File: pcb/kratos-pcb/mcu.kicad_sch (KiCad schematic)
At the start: 1 part, among them U1 ESP32-DEVKIT-V1

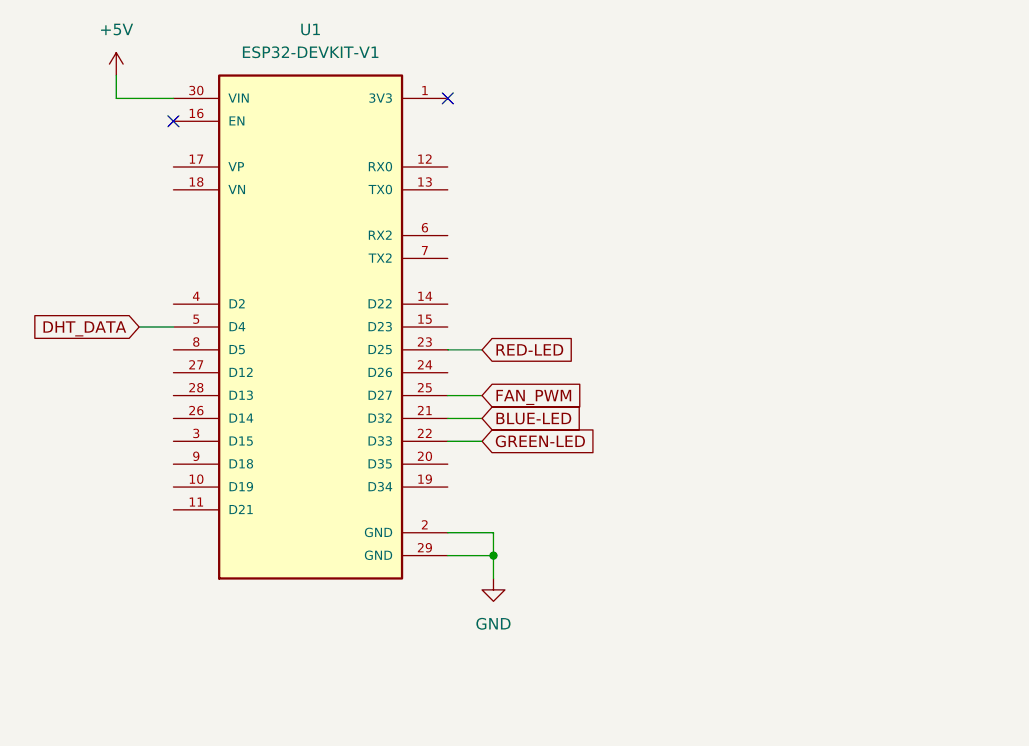
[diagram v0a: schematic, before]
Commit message: ### added
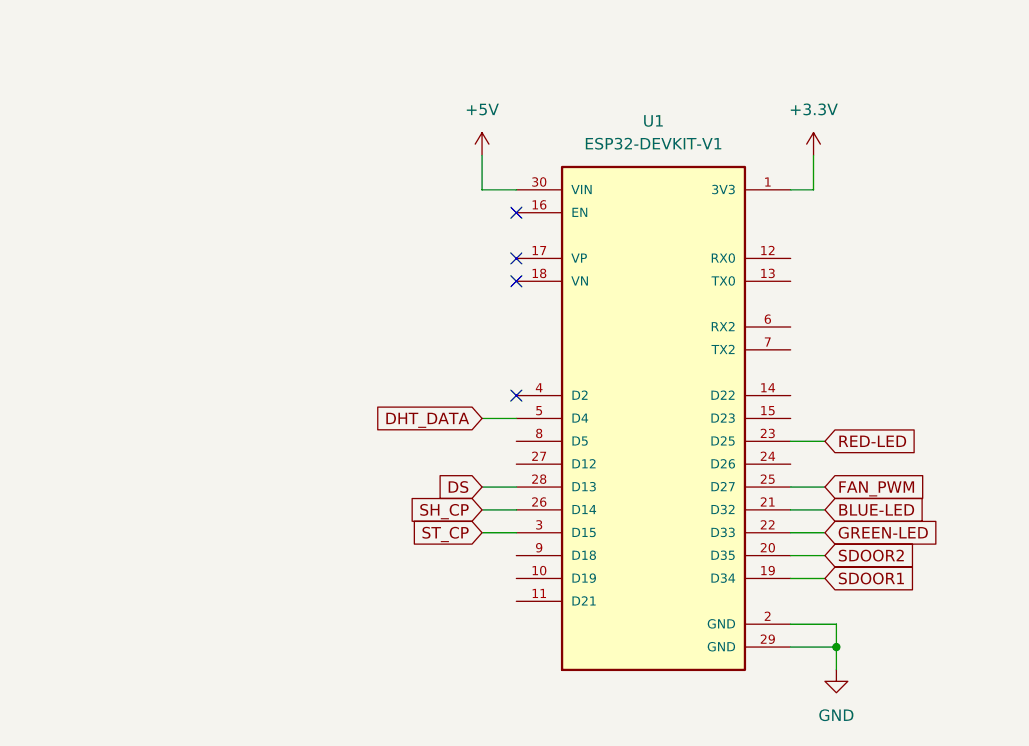
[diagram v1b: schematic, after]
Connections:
- net +3.3V: now reaches U1.1 (3V3)
- net SDOOR1: now reaches U1.19 (D34)
- net SDOOR2: now reaches U1.20 (D35)
- net SH_CP: now reaches U1.26 (D14)
- net DS: now reaches U1.28 (D13)
- net ST_CP: now reaches U1.3 (D15)
- no-connect marks 2 -> 4
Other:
- moved on the sheet: U1

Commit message: ### update     - kicad schematic
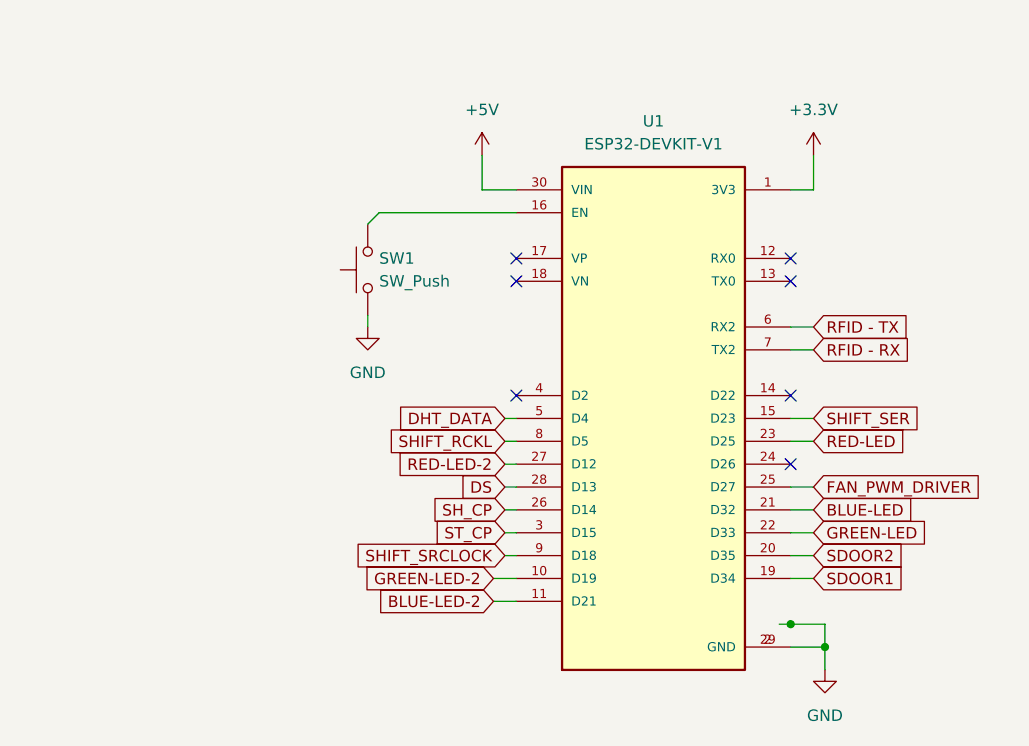
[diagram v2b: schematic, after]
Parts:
- added SW1: SW_Push, Button_Switch_THT:SW_PUSH_6mm_H4.3mm, symbol Switch:SW_Push
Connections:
- net GND: now also SW1.1
- net GREEN-LED-2: now reaches U1.10 (D19)
- net BLUE-LED-2: now reaches U1.11 (D21)
- net SHIFT_SER: now reaches U1.15 (D23)
- net at U1.16 (EN): now also SW1.2
- net RED-LED-2: now reaches U1.27 (D12)
- net RFID - TX: now reaches U1.6 (RX2)
- net RFID - RX: now reaches U1.7 (TX2)
- net SHIFT_RCKL: now reaches U1.8 (D5)
- net SHIFT_SRCLOCK: now reaches U1.9 (D18)
- net FAN_PWM renamed FAN_PWM_DRIVER
- no-connect marks 4 -> 7

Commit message: kicad
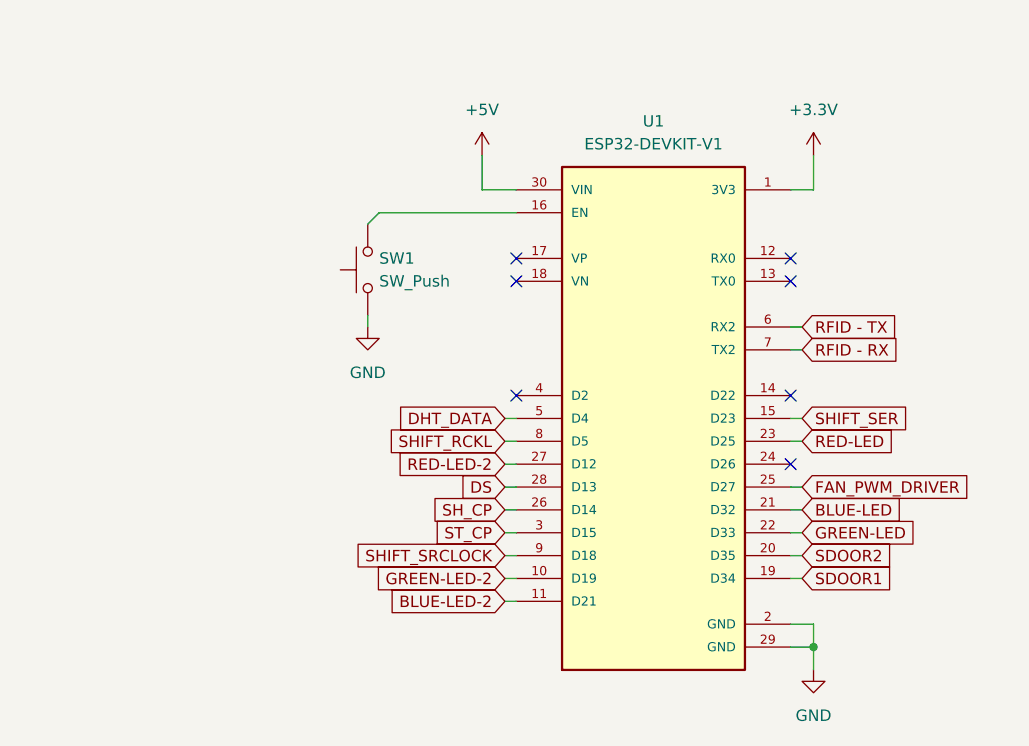
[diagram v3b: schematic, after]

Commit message: ### MODIFY
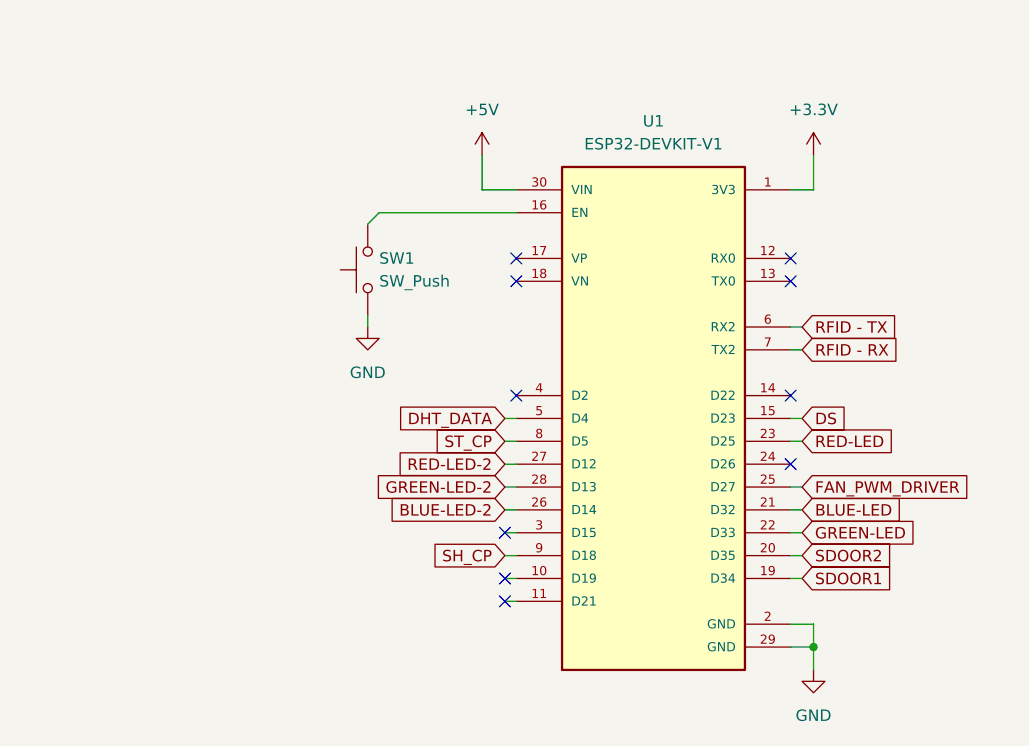
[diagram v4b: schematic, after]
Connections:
- net SHIFT_RCKL is gone; now on net ST_CP: U1.8 (D5)
- net SHIFT_SER is gone; now on net DS: U1.15 (D23)
- net SHIFT_SRCLOCK is gone; now on net SH_CP: U1.9 (D18)
- net BLUE-LED-2: now also U1.26 (D14); no longer U1.11 (D21)
- net DS: no longer U1.28 (D13)
- net GREEN-LED-2: now also U1.28 (D13); no longer U1.10 (D19)
- net SH_CP: no longer U1.26 (D14)
- net ST_CP: no longer U1.3 (D15)
- no-connect marks 7 -> 10
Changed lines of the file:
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@@
   (no_connect (at 158.75 101.6))
   (no_connect (at 128.27 78.74))
+  (no_connect (at 127 109.22))
+  (no_connect (at 127 114.3))
+  (no_connect (at 127 116.84))
   (no_connect (at 158.75 78.74))
   (no_connect (at 128.27 81.28))
@@
     (stroke (width 0) (type default))
   )
-  (global_label "SHIFT_SER" (shape input) (at 160.02 96.52 0) (fields_autoplaced)
-    (effects (font (size 1.27 1.27)) (justify left))
-    (property "Intersheetrefs" "${INTERSHEET_REFS}" (at 172.8023 96.52 0)
-      (effects (font (size 1.27 1.27)) (justify left) hide)
-    )
-  )
   (global_label "SDOOR2" (shape input) (at 160.02 111.76 0) (fields_autoplaced)
     (effects (font (size 1.27 1.27)) (justify left))
@@
     )
   )
-  (global_label "GREEN-LED-2" (shape input) (at 127 114.3 180) (fields_autoplaced)
+  (global_label "SH_CP" (shape input) (at 127 111.76 180) (fields_autoplaced)
     (effects (font (size 1.27 1.27)) (justify right))
-    (property "Intersheetrefs" "${INTERSHEET_REFS}" (at 110.0449 114.3 0)
+    (property "Intersheetrefs" "${INTERSHEET_REFS}" (at 117.9672 111.76 0)
       (effects (font (size 1.27 1.27)) (justify right) hide)
     )
   )
-  (global_label "SH_CP" (shape input) (at 127 106.68 180) (fields_autoplaced)
+  (global_label "BLUE-LED-2" (shape input) (at 127 106.68 180) (fields_autoplaced)
     (effects (font (size 1.27 1.27)) (justify right))
-    (property "Intersheetrefs" "${INTERSHEET_REFS}" (at 117.9672 106.68 0)
+    (property "Intersheetrefs" "${INTERSHEET_REFS}" (at 111.4358 106.68 0)
       (effects (font (size 1.27 1.27)) (justify right) hide)
     )
   )
-  (global_label "BLUE-LED-2" (shape input) (at 127 116.84 180) (fields_autoplaced)
+  (global_label "GREEN-LED-2" (shape input) (at 127 104.14 180) (fields_autoplaced)
     (effects (font (size 1.27 1.27)) (justify right))
-    (property "Intersheetrefs" "${INTERSHEET_REFS}" (at 111.4358 116.84 0)
+    (property "Intersheetrefs" "${INTERSHEET_REFS}" (at 110.0449 104.14 0)
       (effects (font (size 1.27 1.27)) (justify right) hide)
     )
@@
     )
   )
-  (global_label "SHIFT_SRCLOCK" (shape input) (at 127 111.76 180) (fields_autoplaced)
+  (global_label "ST_CP" (shape input) (at 127 99.06 180) (fields_autoplaced)
     (effects (font (size 1.27 1.27)) (justify right))
-    (property "Intersheetrefs" "${INTERSHEET_REFS}" (at 109.1981 111.76 0)
+    (property "Intersheetrefs" "${INTERSHEET_REFS}" (at 118.3301 99.06 0)
       (effects (font (size 1.27 1.27)) (justify right) hide)
     )
@@
     (property "Intersheetrefs" "${INTERSHEET_REFS}" (at 172.9233 86.36 0)
       (effects (font (size 1.27 1.27)) (justify left) hide)
-    )
-  )
-  (global_label "ST_CP" (shape input) (at 127 109.22 180) (fields_autoplaced)
-    (effects (font (size 1.27 1.27)) (justify right))
-    (property "Intersheetrefs" "${INTERSHEET_REFS}" (at 118.3301 109.22 0)
-      (effects (font (size 1.27 1.27)) (justify right) hide)
-    )
-  )
-  (global_label "DS" (shape input) (at 127 104.14 180) (fields_autoplaced)
-    (effects (font (size 1.27 1.27)) (justify right))
-    (property "Intersheetrefs" "${INTERSHEET_REFS}" (at 121.5353 104.14 0)
-      (effects (font (size 1.27 1.27)) (justify right) hide)
     )
   )
@@
     )
   )
+  (global_label "RED-LED" (shape input) (at 160.02 99.06 0) (fields_autoplaced)
+    (effects (font (size 1.27 1.27)) (justify left))
+    (property "Intersheetrefs" "${INTERSHEET_REFS}" (at 171.7137 99.06 0)
+      (effects (font (size 1.27 1.27)) (justify left) hide)
+    )
+  )
   (global_label "GREEN-LED" (shape input) (at 160.02 109.22 0) (fields_autoplaced)
     (effects (font (size 1.27 1.27)) (justify left))
@@
     )
   )
-  (global_label "RED-LED" (shape input) (at 160.02 99.06 0) (fields_autoplaced)
+  (global_label "DS" (shape input) (at 160.02 96.52 0) (fields_autoplaced)
     (effects (font (size 1.27 1.27)) (justify left))
-    (property "Intersheetrefs" "${INTERSHEET_REFS}" (at 171.7137 99.06 0)
+    (property "Intersheetrefs" "${INTERSHEET_REFS}" (at 165.4847 96.52 0)
       (effects (font (size 1.27 1.27)) (justify left) hide)
     )
@@
     )
   )
-  (global_label "SHIFT_RCKL" (shape input) (at 127 99.06 180) (fields_autoplaced)
-    (effects (font (size 1.27 1.27)) (justify right))
-    (property "Intersheetrefs" "${INTERSHEET_REFS}" (at 113.0081 99.06 0)
-      (effects (font (size 1.27 1.27)) (justify right) hide)
-    )
-  )

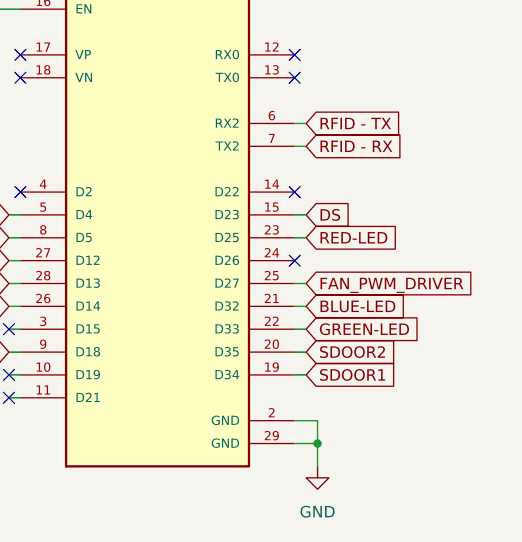
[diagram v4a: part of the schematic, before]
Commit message: ### added
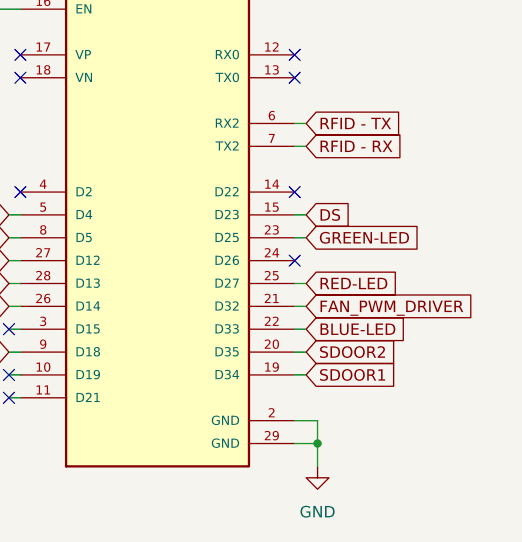
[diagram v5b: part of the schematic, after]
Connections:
- net BLUE-LED: now also U1.22 (D33); no longer U1.21 (D32)
- net FAN_PWM_DRIVER: now also U1.21 (D32); no longer U1.25 (D27)
- net GREEN-LED: now also U1.23 (D25); no longer U1.22 (D33)
- net RED-LED: now also U1.25 (D27); no longer U1.23 (D25)
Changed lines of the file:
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@@
+    )
+  )
+  (global_label "RED-LED" (shape input) (at 160.02 104.14 0) (fields_autoplaced)
+    (effects (font (size 1.27 1.27)) (justify left))
+    (property "Intersheetrefs" "${INTERSHEET_REFS}" (at 171.7137 104.14 0)
+      (effects (font (size 1.27 1.27)) (justify left) hide)
+    )
+  )
+  (global_label "FAN_PWM_DRIVER" (shape input) (at 160.02 106.68 0) (fields_autoplaced)
+    (effects (font (size 1.27 1.27)) (justify left))
+    (property "Intersheetrefs" "${INTERSHEET_REFS}" (at 179.2733 106.68 0)
+      (effects (font (size 1.27 1.27)) (justify left) hide)
     )
   )
@@
     )
   )
-  (global_label "FAN_PWM_DRIVER" (shape input) (at 160.02 104.14 0) (fields_autoplaced)
+  (global_label "GREEN-LED" (shape input) (at 160.02 99.06 0) (fields_autoplaced)
     (effects (font (size 1.27 1.27)) (justify left))
-    (property "Intersheetrefs" "${INTERSHEET_REFS}" (at 179.2733 104.14 0)
+    (property "Intersheetrefs" "${INTERSHEET_REFS}" (at 174.1932 99.06 0)
       (effects (font (size 1.27 1.27)) (justify left) hide)
     )
@@
     )
   )
-  (global_label "RED-LED" (shape input) (at 160.02 99.06 0) (fields_autoplaced)
-    (effects (font (size 1.27 1.27)) (justify left))
-    (property "Intersheetrefs" "${INTERSHEET_REFS}" (at 171.7137 99.06 0)
-      (effects (font (size 1.27 1.27)) (justify left) hide)
-    )
-  )
-  (global_label "GREEN-LED" (shape input) (at 160.02 109.22 0) (fields_autoplaced)
-    (effects (font (size 1.27 1.27)) (justify left))
-    (property "Intersheetrefs" "${INTERSHEET_REFS}" (at 174.1932 109.22 0)
-      (effects (font (size 1.27 1.27)) (justify left) hide)
-    )
-  )
   (global_label "DS" (shape input) (at 160.02 96.52 0) (fields_autoplaced)
     (effects (font (size 1.27 1.27)) (justify left))
@@
     )
   )
-  (global_label "BLUE-LED" (shape input) (at 160.02 106.68 0) (fields_autoplaced)
+  (global_label "BLUE-LED" (shape input) (at 160.02 109.22 0) (fields_autoplaced)
     (effects (font (size 1.27 1.27)) (justify left))
-    (property "Intersheetrefs" "${INTERSHEET_REFS}" (at 172.8023 106.68 0)
+    (property "Intersheetrefs" "${INTERSHEET_REFS}" (at 172.8023 109.22 0)
       (effects (font (size 1.27 1.27)) (justify left) hide)
     )
